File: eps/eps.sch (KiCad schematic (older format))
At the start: 67 parts, among them Q1 IRF7404, Q10 2N7002, Q11 IRF7404, Q12 2N7002, Q13 IRF7404, Q14 2N7002, Q15 IRF7404, Q16 IRF7404, Q17 IRF7404, Q18 IRF7404, Q19 IRF7404, Q2 2N7002, Q20 2N7002, Q21 IRF7404, Q22 2N7002, Q23 IRF7404, Q24 2N7002, Q3 IRF7404, Q4 2N7002, Q5 IRF7404, Q6 2N7002, Q7 IRF7404, Q8 2N7002, Q9 IRF7404, U1 ADP2302ARDZ-3.3, U2 ADP2303ARDZ-5.0, U3 CS5172EDR8G

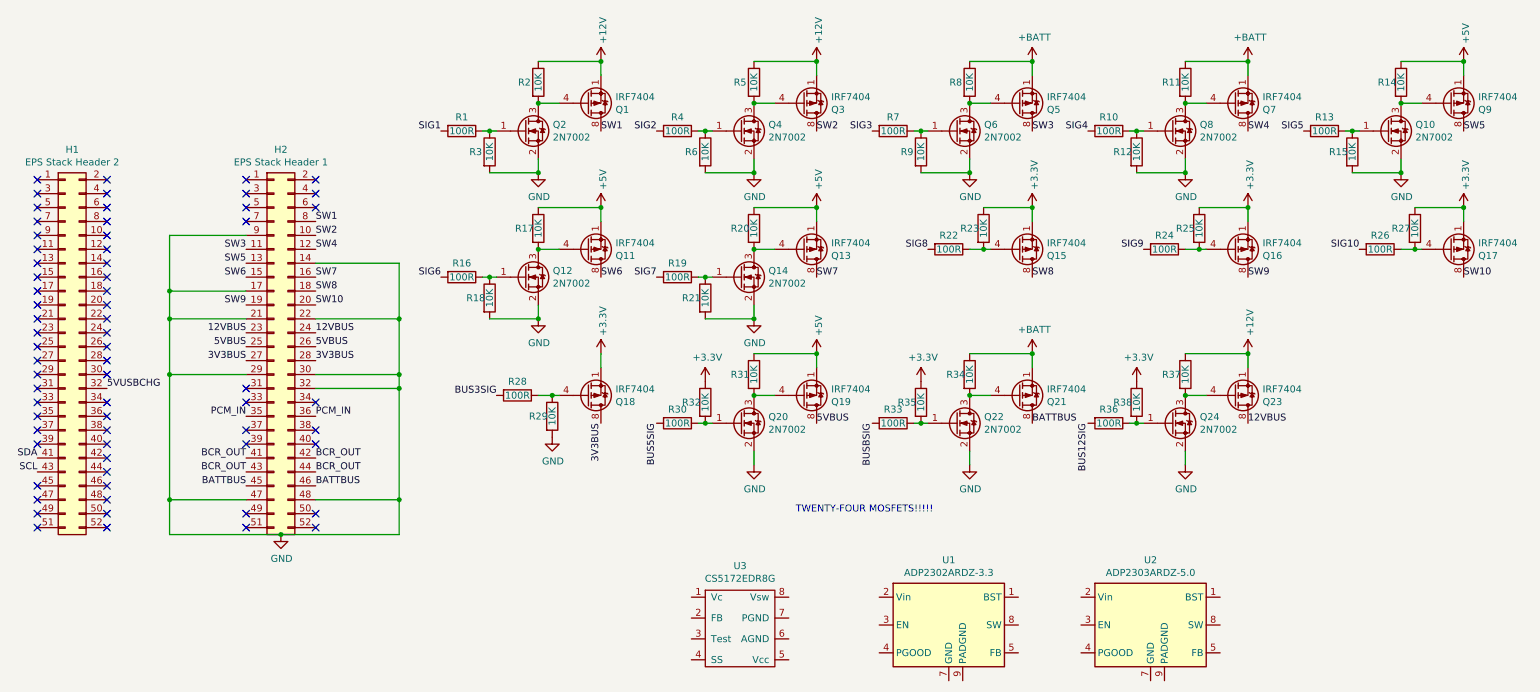
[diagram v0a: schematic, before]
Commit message: organization
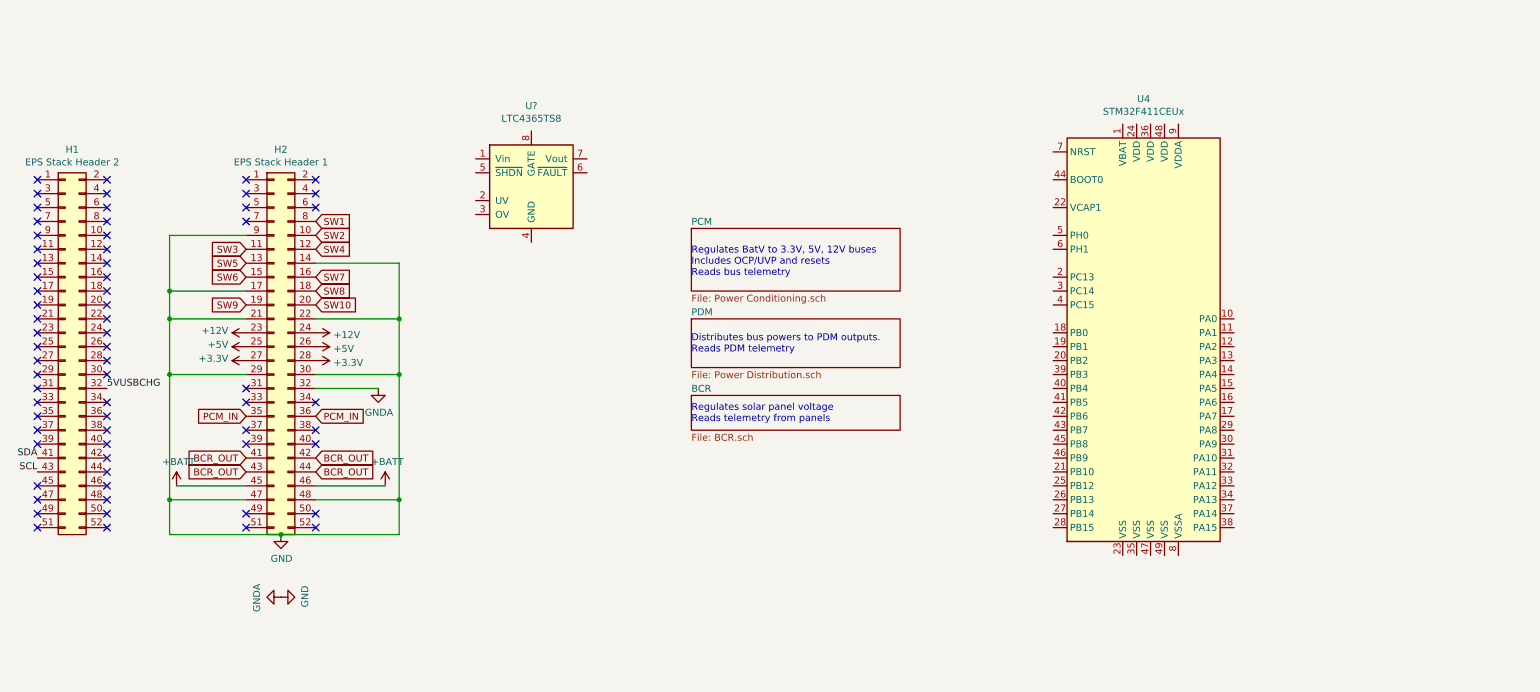
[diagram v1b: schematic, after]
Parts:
- removed Q1, Q11, Q13, Q15, Q16, Q17, Q18, Q19, Q21, Q23, Q3, Q5, Q7, Q9: IRF7404, Package_SO:SOIC-8_3.9x4.9mm_P1.27mm, symbol Transistor_FET:IRF7404
- removed Q10, Q12, Q14, Q2, Q20, Q22, Q24, Q4, Q6, Q8: 2N7002, Package_TO_SOT_SMD:SOT-23, symbol Transistor_FET:2N7002
- removed R1, R10, R13, R16, R19, R22, R24, R26, R28, R30, R33, R36, R4, R7: 100R, symbol Device:R
- removed R11, R12, R14, R15, R17, R18, R2, R20, R21, R23, R25, R27, R29, R3, R31, R32, R34, R35, R37, R38, R5, R6, R8, R9: 10K, symbol Device:R
- removed U1: ADP2302ARDZ-3.3, Package_SO:SOIC-8-1EP_3.9x4.9mm_P1.27mm_EP2.29x3mm, symbol Regulator_Switching:ADP2302ARDZ-3.3
- removed U2: ADP2303ARDZ-5.0, Package_SO:SOIC-8-1EP_3.9x4.9mm_P1.27mm_EP2.29x3mm, symbol Regulator_Switching:ADP2303ARDZ-5.0
- removed U3: CS5172EDR8G, symbol epslib:CS5172EDR8G
- added U4: STM32F411CEUx, Package_DFN_QFN:QFN-48-1EP_7x7mm_P0.5mm_EP5.6x5.6mm, symbol MCU_ST_STM32F4:STM32F411CEUx
- added U?: LTC4365TS8, symbol Power_Management:LTC4365TS8
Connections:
- net 12VBUS is gone; now on net +12V: H2.23 (Pin_23), H2.24 (Pin_24)
- net 3V3BUS is gone; now on net +3V3: H2.27 (Pin_27), H2.28 (Pin_28)
- net 5VBUS is gone; now on net +5V: H2.25 (Pin_25), H2.26 (Pin_26)
- net BATTBUS is gone; now on net +BATT: H2.45 (Pin_45), H2.46 (Pin_46)
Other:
- note added: "Distributes bus powers to PDM outputs. \nReads PDM telemetry\n"
- note added: "Regulates BatV to 3.3V, 5V, 12V buses\nIncludes OCP/UVP and resets\nReads bus telemetry"
- note added: "Regulates solar panel voltage\nReads telemetry from panels\n"
- note removed: "TWENTY-FOUR MOSFETS!!!!!"
